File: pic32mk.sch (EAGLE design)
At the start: 1 part, among them IC1 PIC32MK1024MCF100-I_PT

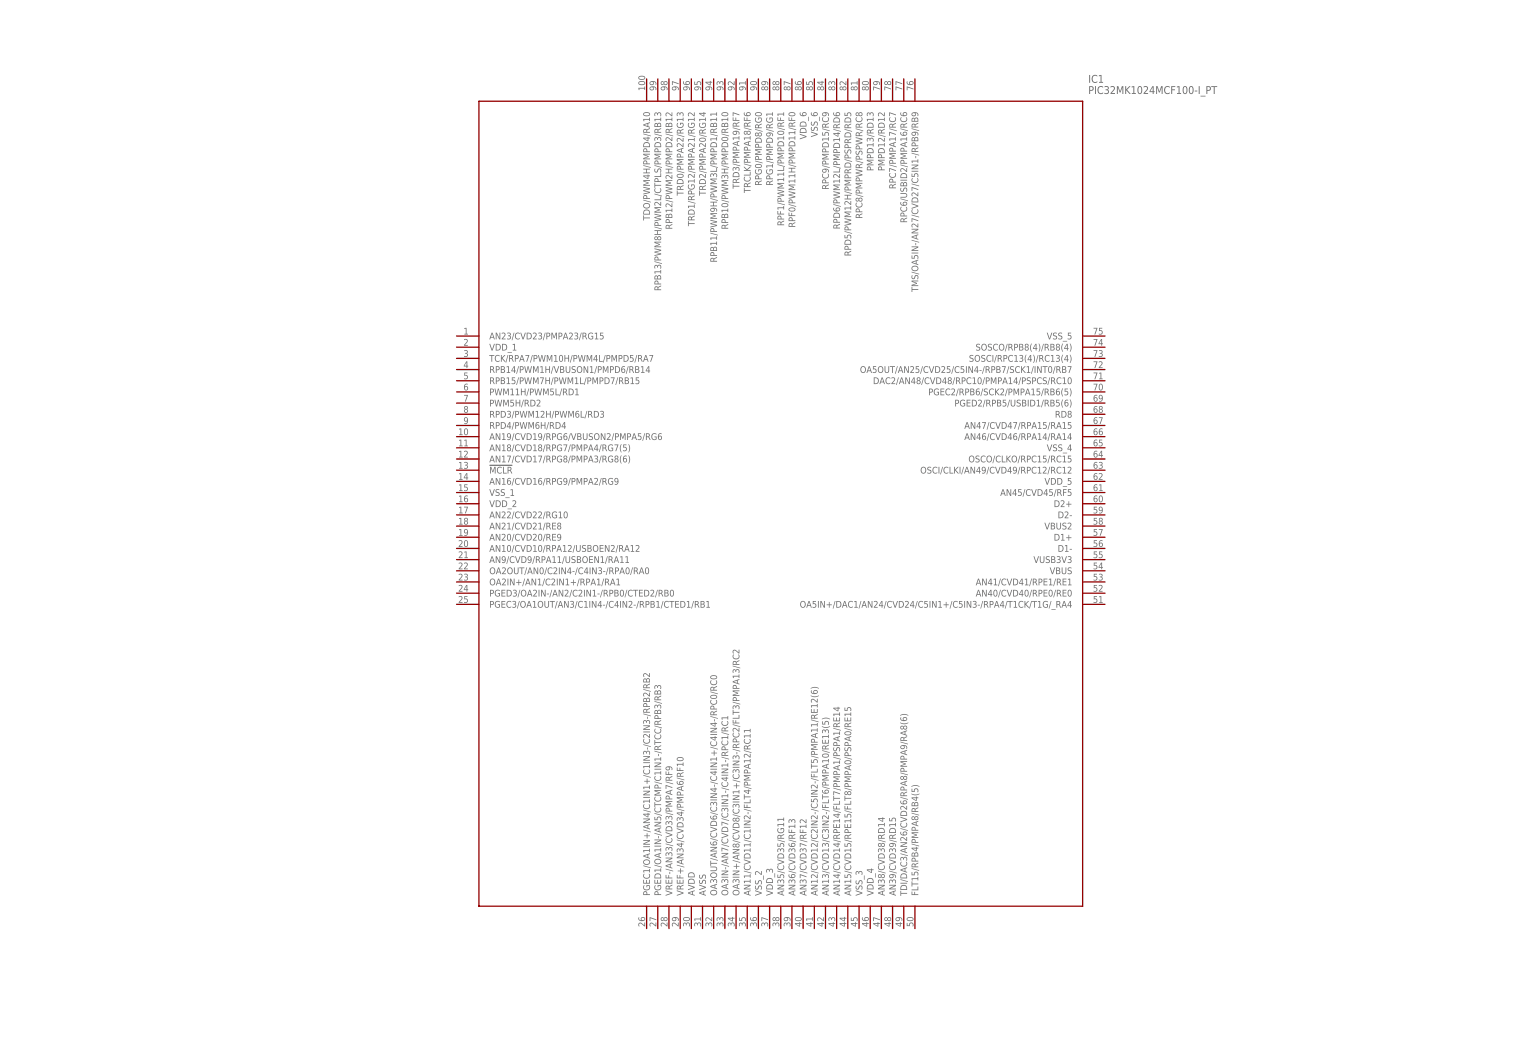
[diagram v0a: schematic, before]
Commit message: up
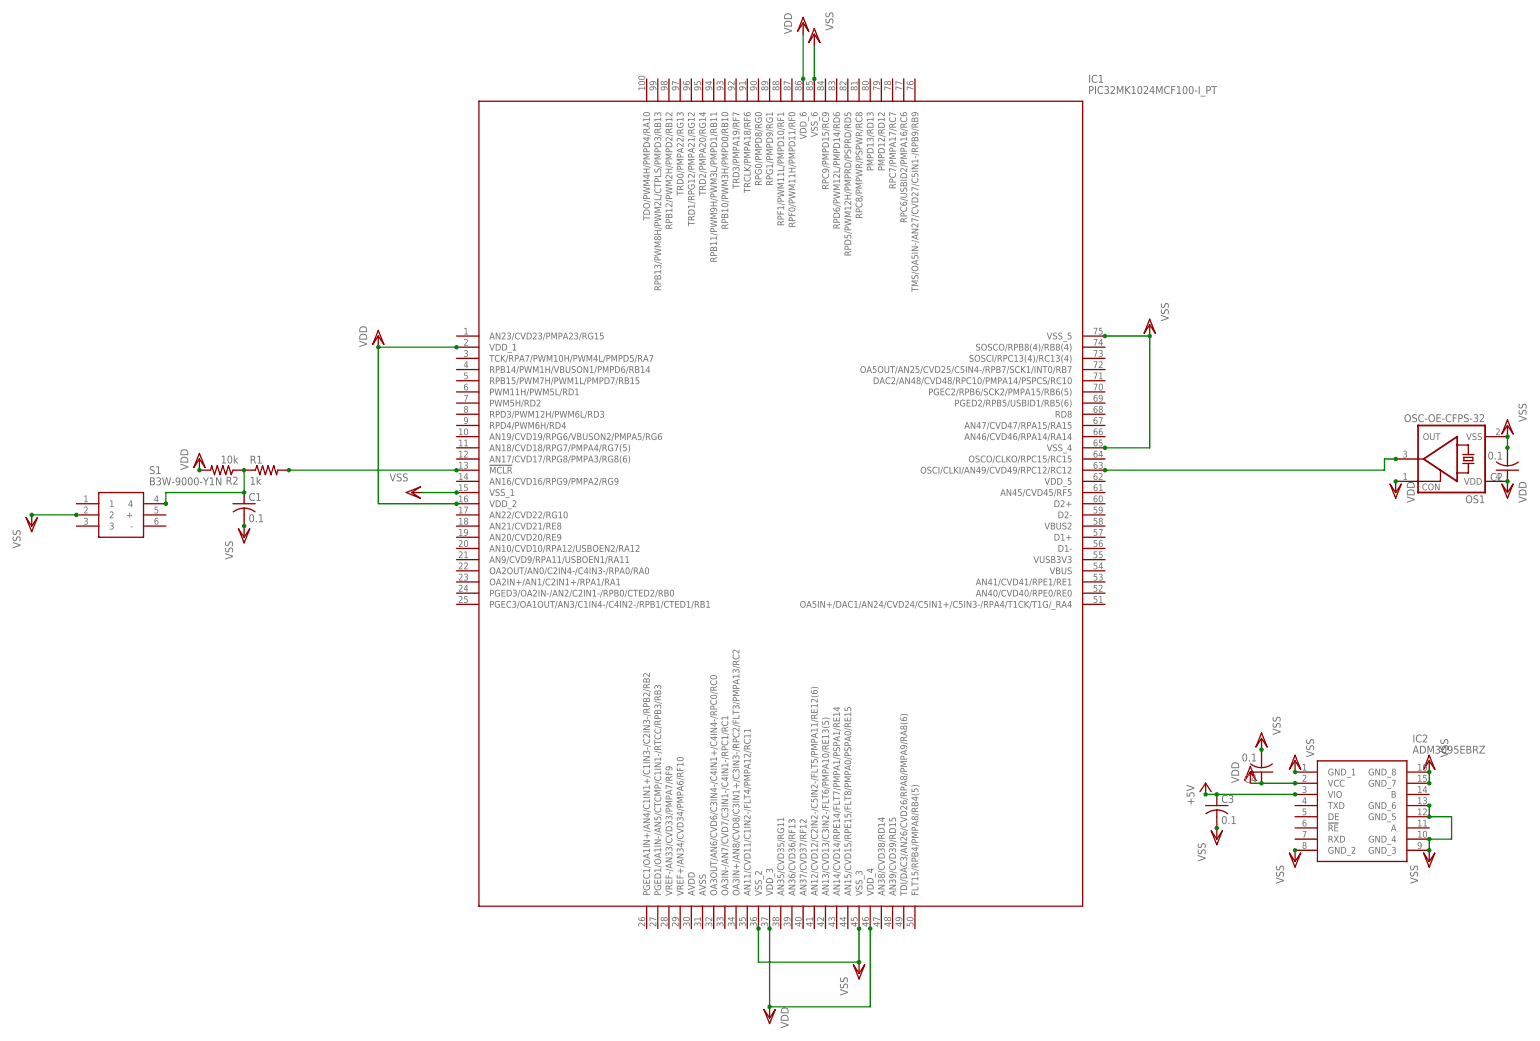
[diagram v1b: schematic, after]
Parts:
- added C1, C2, C3, C4: 0.1, rcl:C-USC0805
- added IC2: ADM3095EBRZ, SamacSys_Parts:ADM3095EBRZ
- added OS1: OSC-OE-CFPS-32, IQD-Frequency-Products:OSC-OE-CFPS-32
- added R1: 1k, rcl:R-US_M0805
- added R2: 10k, rcl:R-US_M0805
- added S1: B3W-9000-Y1N, B3W-9000-Y1N:B3W-9000-Y1N
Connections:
- new net +5V: C3.1, IC2.VIO
- new net N$1: C1.1, R1.1, R2.1, S1.4
- new net N$2: IC1.!MCLR, R1.2
- new net N$3: IC1.OSCI/CLKI/AN49/CVD49/RPC12/RC12, OS1.OUT
- new net VDD: C2.1, C4.1, IC1.VDD_1, IC1.VDD_2, IC1.VDD_3, IC1.VDD_4, IC1.VDD_6, IC2.VCC, OS1.CON, OS1.VDD, R2.2
- new net VSS: C1.2, C2.2, C3.2, C4.2, IC1.VSS_1, IC1.VSS_2, IC1.VSS_3, IC1.VSS_4, IC1.VSS_5, IC1.VSS_6, IC2.GND_1, IC2.GND_2, IC2.GND_3, IC2.GND_4, IC2.GND_5, IC2.GND_6, IC2.GND_7, IC2.GND_8, OS1.VSS, S1.2
